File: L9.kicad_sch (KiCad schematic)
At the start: 38 parts

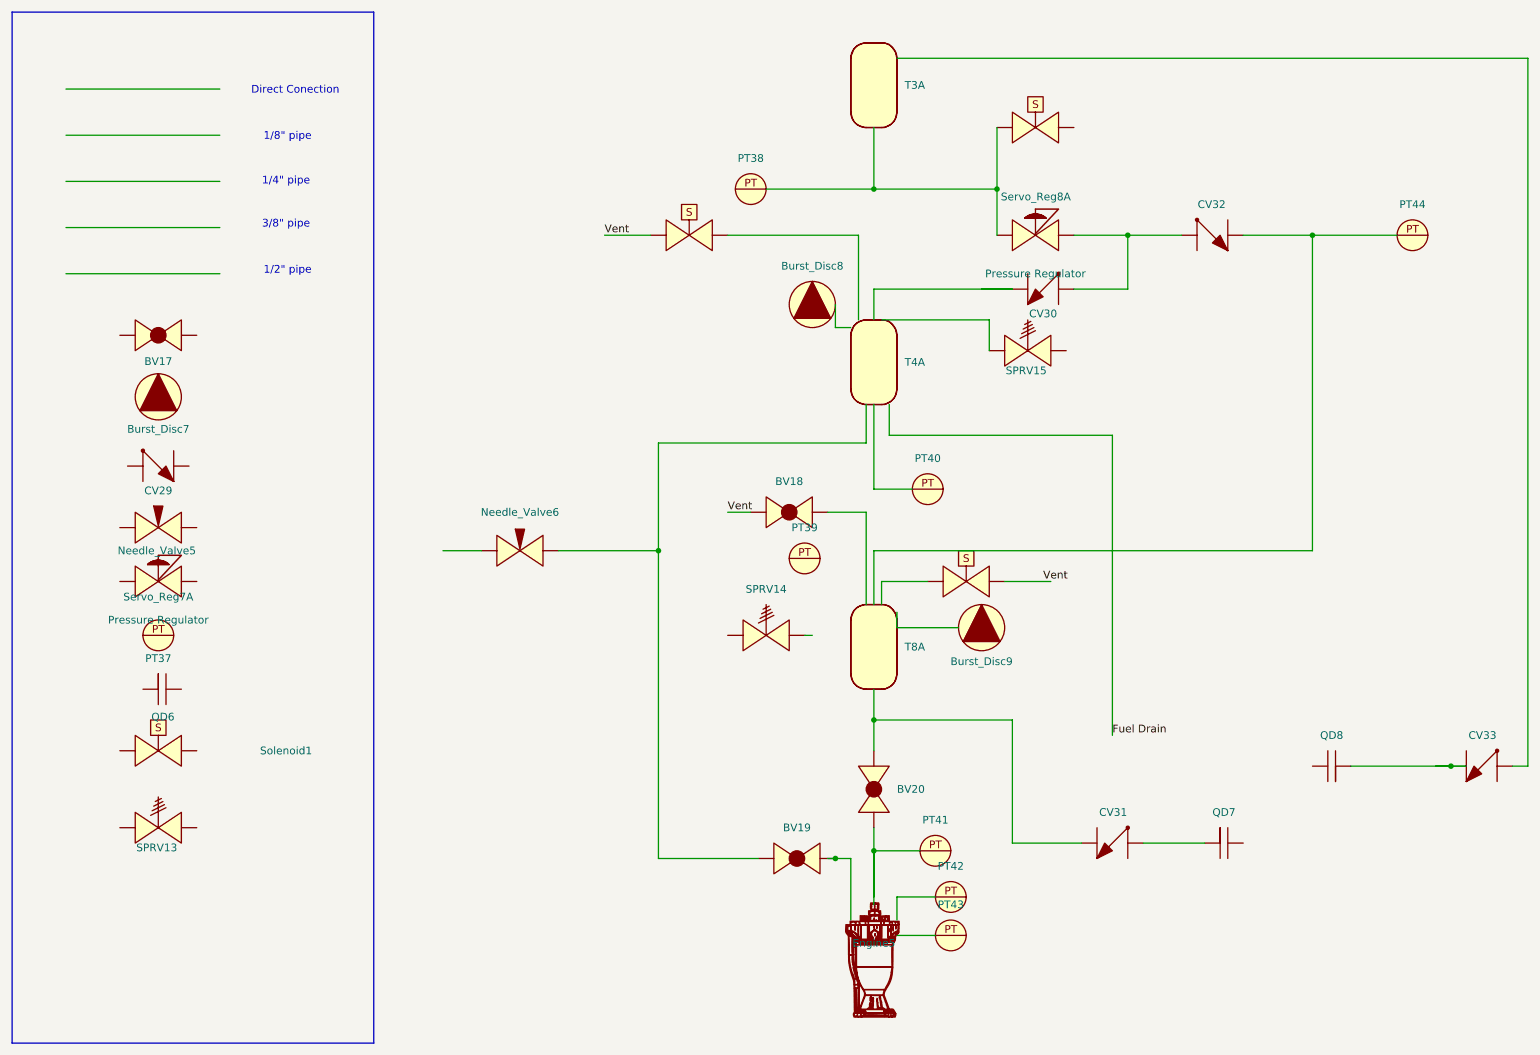
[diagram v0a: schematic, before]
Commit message: Formatiing
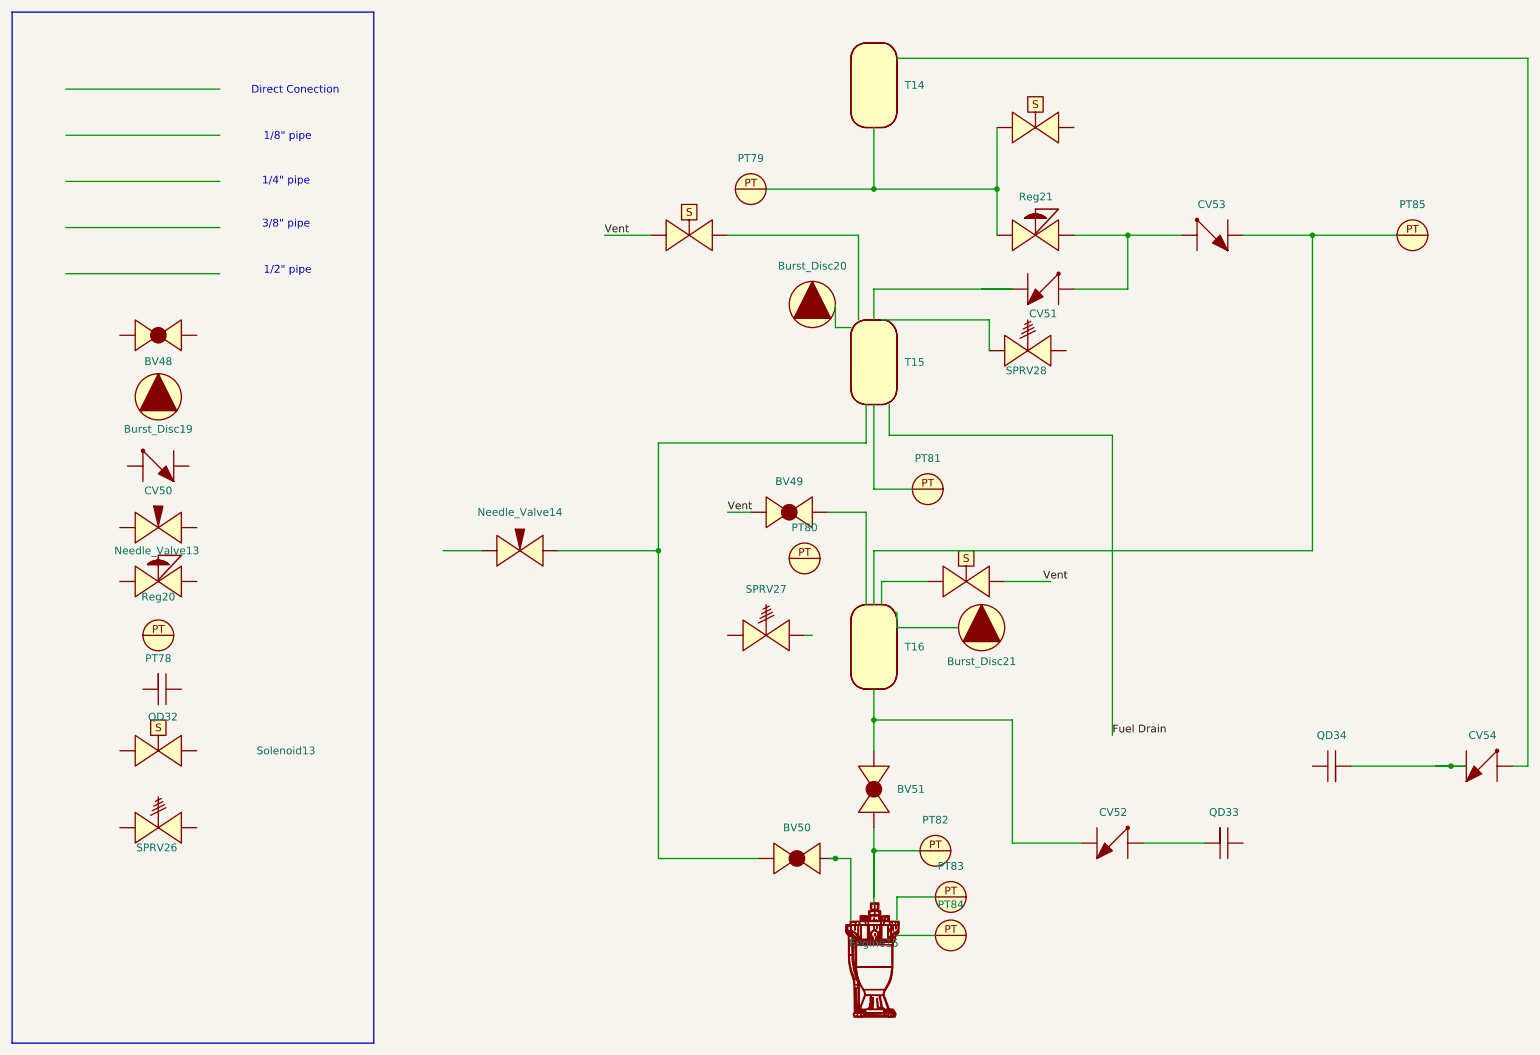
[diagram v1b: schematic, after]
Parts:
- renumbered BV17 to BV48, BV18 to BV49, BV19 to BV50, BV20 to BV51, Burst_Disc7 to Burst_Disc19, Burst_Disc8 to Burst_Disc20, Burst_Disc9 to Burst_Disc21, CV29 to CV50, CV30 to CV51, CV31 to CV52, CV32 to CV53, CV33 to CV54, Engine5 to Engine15, Needle_Valve5 to Needle_Valve13, Needle_Valve6 to Needle_Valve14, PT37 to PT78, PT38 to PT79, PT39 to PT80, PT40 to PT81, PT41 to PT82, PT42 to PT83, PT43 to PT84, PT44 to PT85, QD6 to QD32, QD7 to QD33, QD8 to QD34, Servo_Reg7 to Reg20, Servo_Reg8 to Reg21, SPRV13 to SPRV26, SPRV14 to SPRV27, SPRV15 to SPRV28, Solenoid1 to Solenoid13, Solenoid2 to Solenoid14, Solenoid3 to Solenoid15, Solenoid4 to Solenoid16, T3 to T14, T4 to T15, T8 to T16
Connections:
- net at QD33.: now also CV52.
- net at CV52.: now also BV51., T16.; no longer QD33.
- net at PT85.: now also CV53., T16.
- net at CV54.: now also QD34.
- net at QD34.: no longer CV54.
- net at Engine15.: now also BV51., PT82.
- net at BV50.: now also Needle_Valve14.; no longer Engine15.
- net at PT83.: no longer Engine15.
- new net: CV51., CV53., Reg21.
- new net: PT79., Reg21., Solenoid16., T14.
- new net: BV50., Engine15.
- new net: Engine15., PT83.
- now unconnected: PT79., PT82., Solenoid16., T14.
